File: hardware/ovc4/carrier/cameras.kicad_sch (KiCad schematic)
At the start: 7 parts, among them U1 Jetson_Nano, U12 PICAM, U13 PICAM, U14 PICAM, U15 PICAM, U16 PICAM, U17 PICAM

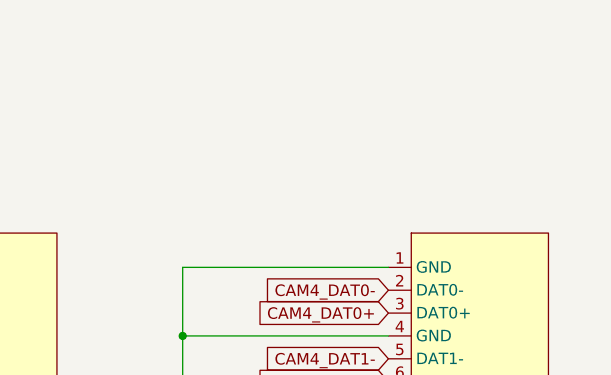
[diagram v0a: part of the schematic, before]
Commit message: Finished first iteration of placement and routing
Signed-off-by: Luca Della Vedova <luca@openrobotics.org>
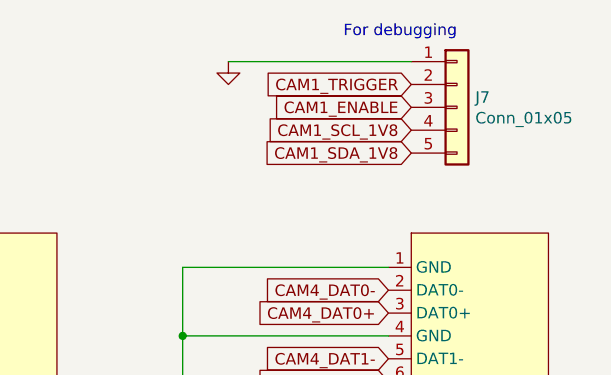
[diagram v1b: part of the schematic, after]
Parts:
- added J7: Conn_01x05, Connector_PinHeader_2.54mm:PinHeader_1x05_P2.54mm_Vertical, symbol Connector_Generic:Conn_01x05
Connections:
- net CAM1_ENABLE: now also J7.3 (Pin_3)
- net CAM1_SCL_1V8: now also J7.4 (Pin_4)
- net CAM1_SDA_1V8: now also J7.5 (Pin_5)
- net CAM1_TRIGGER: now also J7.2 (Pin_2)
- net GND: now also J7.1 (Pin_1)
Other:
- note added: "For debugging"
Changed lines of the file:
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@@
   (junction (at 226.06 124.46))
   (junction (at 226.06 132.08))
+  (no_connect (at 39.37 128.27))
+  (no_connect (at 39.37 153.67))
+  (no_connect (at 39.37 138.43))
+  (no_connect (at 39.37 140.97))
+  (no_connect (at 39.37 125.73))
   (no_connect (at 39.37 130.81))
-  (no_connect (at 39.37 138.43))
+  (no_connect (at 39.37 156.21))
   (no_connect (at 39.37 133.35))
-  (no_connect (at 39.37 156.21))
   (no_connect (at 39.37 146.05))
-  (no_connect (at 39.37 153.67))
-  (no_connect (at 39.37 125.73))
-  (no_connect (at 39.37 128.27))
-  (no_connect (at 39.37 140.97))
   (no_connect (at 39.37 148.59))
   (wire (pts (xy 116.84 50.8) (xy 116.84 58.42)))
@@
   (wire (pts (xy 228.6 86.36) (xy 248.92 86.36)))
   (wire (pts (xy 228.6 144.78) (xy 248.92 144.78)))
+  (wire (pts (xy 231.14 27.94) (xy 251.46 27.94)))
   (text "TODO decide how to use only GPIO (or use ENABLE as gpio as well)"
     (at 200.66 25.4 0)
     (effects (font (size 1.27 1.27)) (justify right bottom))
   )
+  (text "For debugging" (at 256.54 25.4 180)
+    (effects (font (size 1.27 1.27)) (justify right bottom))
+  )
   (global_label "CAM0_CLK-" (shape input) (at 39.37 39.37 0)
     (effects (font (size 1.27 1.27)) (justify left))
@@
   )
   (global_label "CAM5_SDA_1V8" (shape input) (at 248.92 142.24 180)
+    (effects (font (size 1.27 1.27)) (justify right))
+  )
+  (global_label "CAM1_TRIGGER" (shape input) (at 251.46 30.48 180)
+    (effects (font (size 1.27 1.27)) (justify right))
+  )
+  (global_label "CAM1_ENABLE" (shape input) (at 251.46 33.02 180)
+    (effects (font (size 1.27 1.27)) (justify right))
+  )
+  (global_label "CAM1_SCL_1V8" (shape input) (at 251.46 35.56 180)
+    (effects (font (size 1.27 1.27)) (justify right))
+  )
+  (global_label "CAM1_SDA_1V8" (shape input) (at 251.46 38.1 180)
     (effects (font (size 1.27 1.27)) (justify right))
   )
@@
     )
   )
+  (symbol (lib_id "power:GND") (at 231.14 27.94 0) (unit 1)
+    (property "Reference" "#PWR0235" (id 0) (at 231.14 34.29 0)
+      (effects (font (size 1.27 1.27)) hide)
+    )
+    (property "Value" "GND" (id 1) (at 231.267 32.3342 0)
+      (effects (font (size 1.27 1.27)) hide)
+    )
+    (property "Footprint" "" (id 2) (at 231.14 27.94 0)
+      (effects (font (size 1.27 1.27)) hide)
+    )
+    (property "Datasheet" "" (id 3) (at 231.14 27.94 0)
+      (effects (font (size 1.27 1.27)) hide)
+    )
+  )
   (symbol (lib_id "power:GND") (at 259.08 91.44 0) (unit 1)
     (property "Reference" "#PWR0192" (id 0) (at 259.08 97.79 0)
@@
       (effects (font (size 1.27 1.27)) hide)
     )
+  )
+  (symbol (lib_id "Connector_Generic:Conn_01x05") (at 256.54 33.02 0) (unit 1)
+    (property "Reference" "J7" (id 0) (at 258.5721 31.9214 0)
+      (effects (font (size 1.27 1.27)) (justify left))
+    )
+    (property "Value" "Conn_01x05" (id 1) (at 258.5721 34.2201 0)
+      (effects (font (size 1.27 1.27)) (justify left))
+    )
+    (property "Footprint" "Connector_PinHeader_2.54mm:PinHeader_1x05_P2.54mm_Vertical" (id 2) (at 256.54 33.02 0)
+      (effects (font (size 1.27 1.27)) hide)
+    )
+    (property "Datasheet" "~" (id 3) (at 256.54 33.02 0)
+      (effects (font (size 1.27 1.27)) hide)
+    )
